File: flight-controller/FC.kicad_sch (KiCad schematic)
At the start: 1 part, among them U2 ESP32-S3-MINI-1

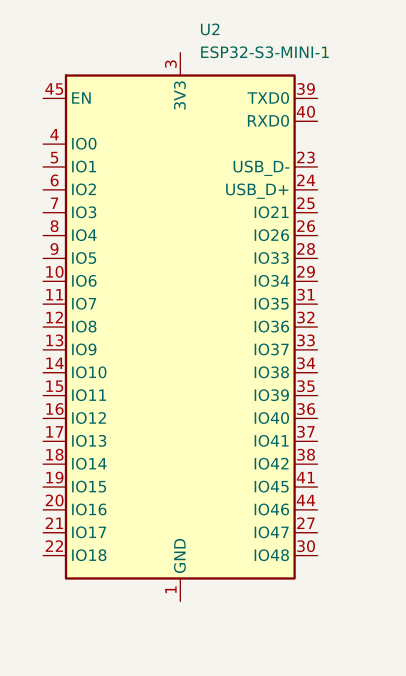
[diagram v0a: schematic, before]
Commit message: clean hierachy
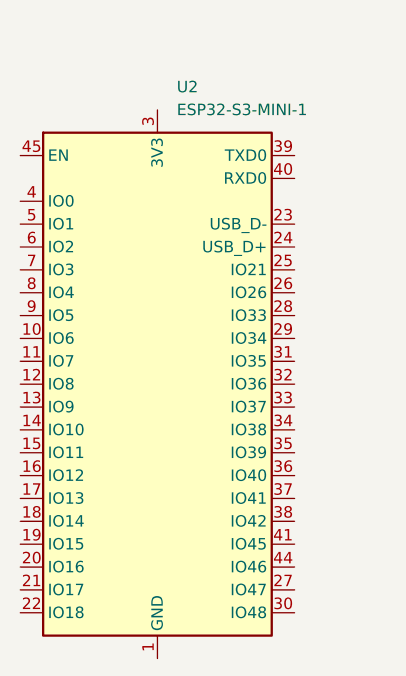
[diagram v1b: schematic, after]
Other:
- moved on the sheet: U2
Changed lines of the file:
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@@
 	(symbol
 		(lib_id "RF_Module:ESP32-S3-MINI-1")
-		(at 80.01 64.77 0)
+		(at 77.47 71.12 0)
 		(unit 1)
 		(body_style 1)
@@
 		(fields_autoplaced yes)
 		(property "Reference" "U2"
-			(at 82.1533 31.75 0)
+			(at 79.6133 38.1 0)
 			(show_name no)
 			(do_not_autoplace no)
@@
 		)
 		(property "Value" "ESP32-S3-MINI-1"
-			(at 82.1533 34.29 0)
+			(at 79.6133 40.64 0)
 			(show_name no)
 			(do_not_autoplace no)
@@
 		)
 		(property "Footprint" "RF_Module:ESP32-S2-MINI-1"
-			(at 95.25 93.98 0)
+			(at 92.71 100.33 0)
 			(hide yes)
 			(show_name no)
@@
 		)
 		(property "Datasheet" "https://www.espressif.com/sites/default/files/documentation/esp32-s3-mini-1_mini-1u_datasheet_en.pdf"
-			(at 80.01 24.13 0)
+			(at 77.47 30.48 0)
 			(hide yes)
 			(show_name no)
@@
 		)
 		(property "Description" "RF Module, ESP32-S3 SoC, Wi-Fi 802.11b/g/n, Bluetooth, BLE, 32-bit, 3.3V, SMD, onboard antenna"
-			(at 80.01 21.59 0)
+			(at 77.47 27.94 0)
 			(hide yes)
 			(show_name no)
@@
 		)
 		(instances
-			(project "Power Board"
+			(project "flight-controller"
 				(path "/e1d5dd76-ec41-4f53-aa0b-5d03fb935d99/ab31c291-e8bf-479a-b3ea-b25df21dfdbf"
 					(reference "U2")
